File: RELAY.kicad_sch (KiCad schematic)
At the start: 36 parts, among them K1 FINDER-36.11, K2 FINDER-36.11, K3 FINDER-36.11, K4 FINDER-36.11, Q1 BC847, Q2 BC847, Q3 BC847, Q4 BC847, U10 LTV-817S, U7 LTV-817S, U8 LTV-817S, U9 LTV-817S

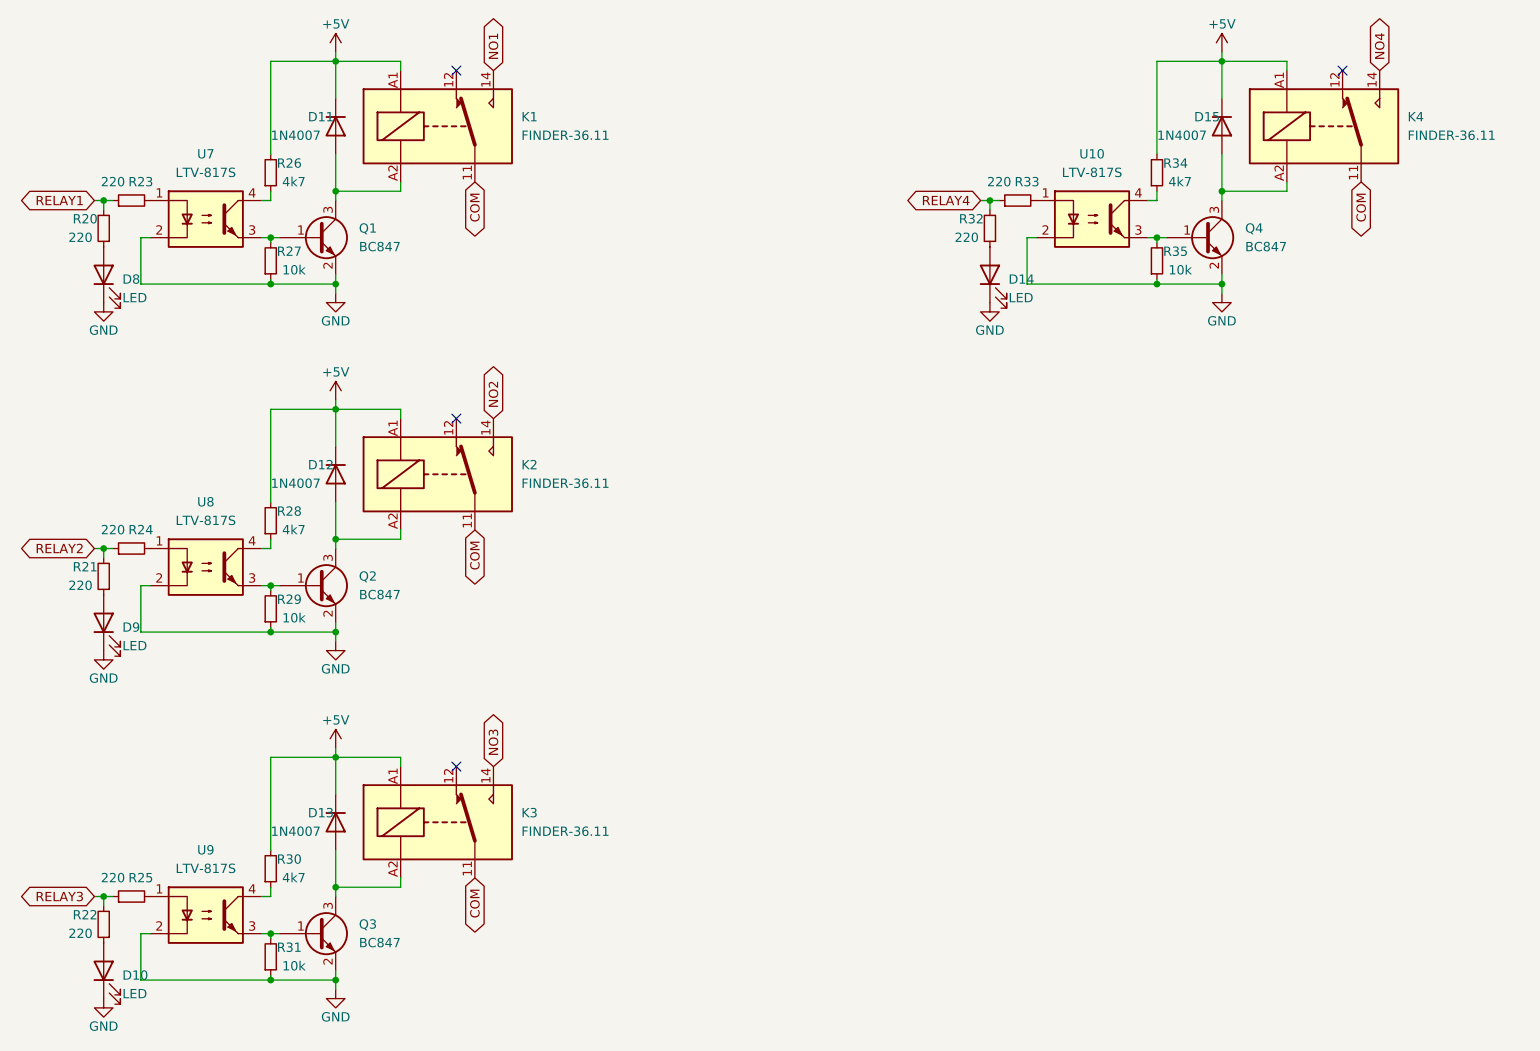
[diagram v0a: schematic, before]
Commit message: Add files via upload
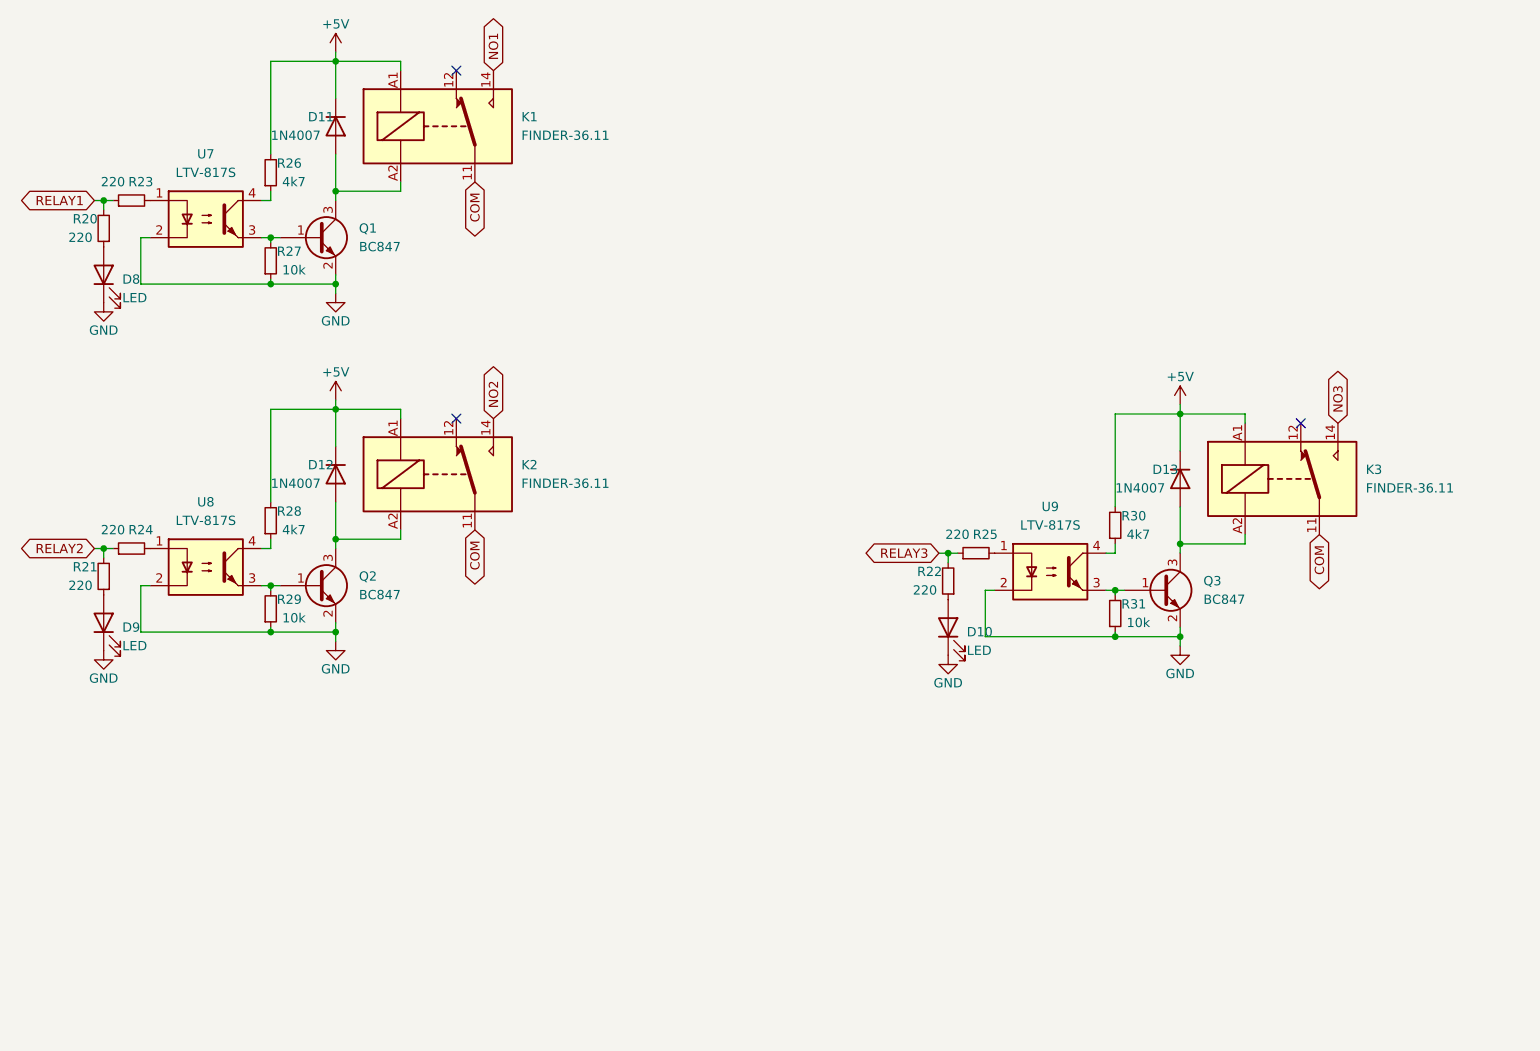
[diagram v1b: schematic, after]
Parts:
- removed D14: LED, LED_SMD:LED_0603_1608Metric, symbol Device:LED
- removed D15: 1N4007, Diode_SMD:D_SOD-123, symbol Diode:1N4148W
- removed K4: FINDER-36.11, Relay_THT:Relay_SPDT_Finder_36.11, symbol Relay:FINDER-36.11
- removed Q4: BC847, Package_TO_SOT_SMD:SOT-23, symbol Transistor_BJT:BC847
- removed R32, R33: 220, Resistor_SMD:R_0603_1608Metric, symbol Device:R_Small
- removed R34: 4k7, Resistor_SMD:R_0603_1608Metric, symbol Device:R_Small
- removed R35: 10k, Resistor_SMD:R_0603_1608Metric, symbol Device:R_Small
- removed U10: LTV-817S, Package_DIP:SMDIP-4_W9.53mm, symbol Isolator:LTV-817S
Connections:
- no-connect marks 4 -> 3
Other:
- moved on the sheet: D10, D13, K3, Q3, R22, R25, R30, R31, U9

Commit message: Add files via upload
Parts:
- D11, D12, D13: footprint Diode_SMD:D_SOD-123 -> Diode_SMD:D_SOD-123F
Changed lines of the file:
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@@
       (effects (font (size 1.27 1.27)) (justify left))
     )
-    (property "Footprint" "Diode_SMD:D_SOD-123" (id 2) (at 95.885 98.425 0)
+    (property "Footprint" "Diode_SMD:D_SOD-123F" (id 2) (at 95.885 98.425 0)
       (effects (font (size 1.27 1.27)) hide)
     )
@@
       (effects (font (size 1.27 1.27)) (justify left))
     )
-    (property "Footprint" "Diode_SMD:D_SOD-123" (id 2) (at 211.455 99.06 0)
+    (property "Footprint" "Diode_SMD:D_SOD-123F" (id 2) (at 211.455 99.06 0)
       (effects (font (size 1.27 1.27)) hide)
     )
@@
       (effects (font (size 1.27 1.27)) (justify left))
     )
-    (property "Footprint" "Diode_SMD:D_SOD-123" (id 2) (at 95.885 50.8 0)
+    (property "Footprint" "Diode_SMD:D_SOD-123F" (id 2) (at 95.885 50.8 0)
       (effects (font (size 1.27 1.27)) hide)
     )
